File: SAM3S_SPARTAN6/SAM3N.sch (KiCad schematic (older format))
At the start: 28 parts, among them U11 ZLDO1117G33TA, X401 12MHz

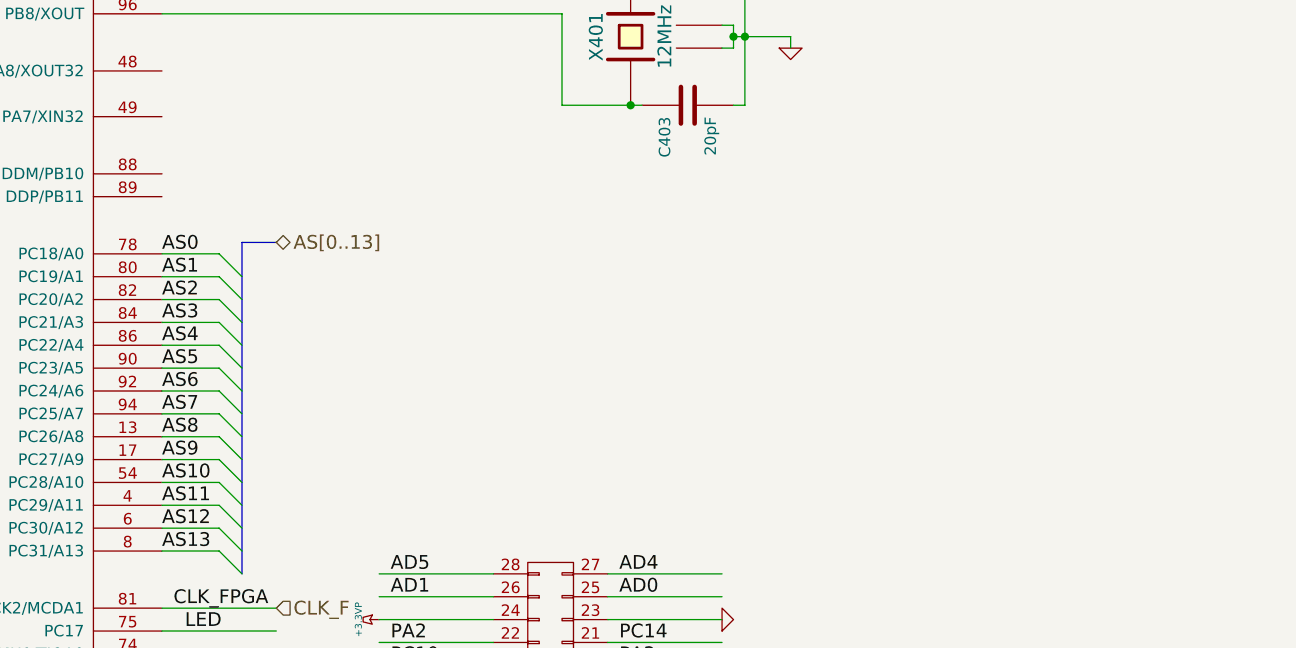
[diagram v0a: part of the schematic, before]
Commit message: Routing
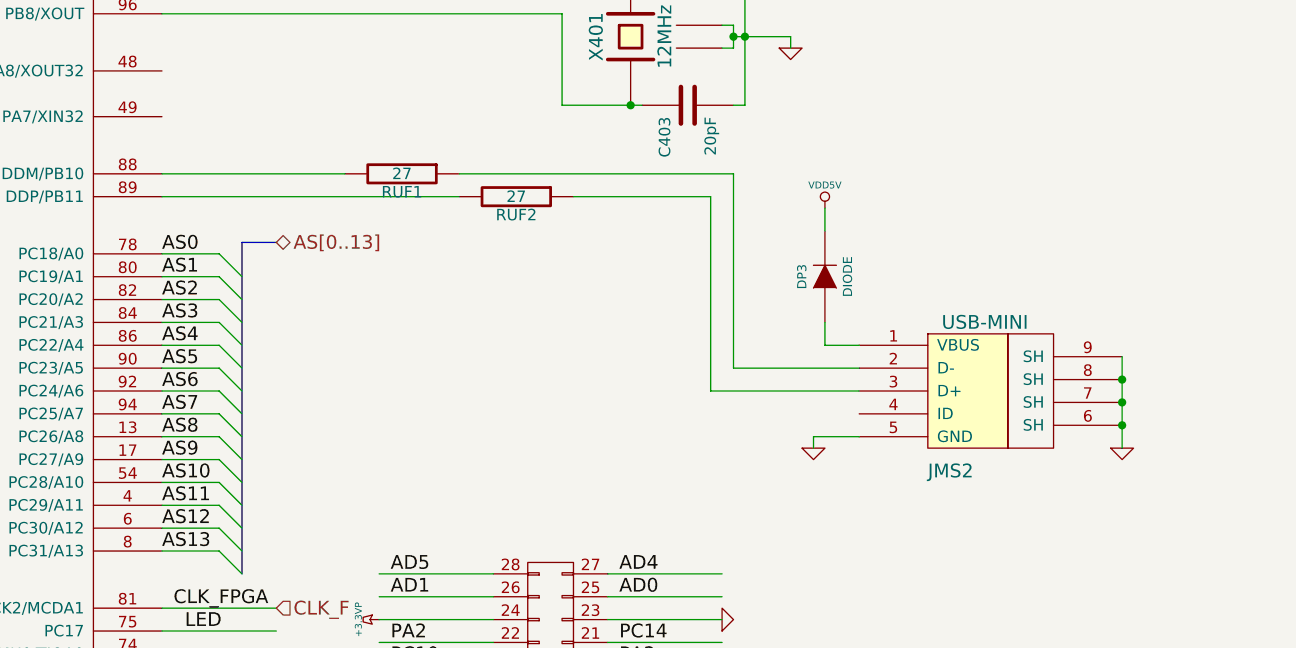
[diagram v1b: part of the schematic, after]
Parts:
- added DP3: DIODE, opendous:SM0603_Opendous, symbol DIODE
- added JMS2: USB-MINI, Connect:USB_Mini-B, symbol USB-MINI
- added RUF1, RUF2: 27, SM0603, symbol R
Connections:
- wire segments 165 -> 180
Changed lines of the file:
@@
 Text HLabel 5400 4600 2    60   Input ~ 0
 CLK_F
+$Comp
+L USB-MINI JMS2
+U 1 1 555B7046
+P 8600 3550
+F 0 "JMS2" H 8350 4000 60  0000 C CNN
+F 1 "USB-MINI" H 8500 3350 60  0000 C CNN
+F 2 "Connect:USB_Mini-B" H 8600 3550 60  0001 C CNN
+F 3 "" H 8600 3550 60  0000 C CNN
+	1    8600 3550
+	1    0    0    1
+$EndComp
+Wire Wire Line
+	7400 3550 7950 3550
+Wire Wire Line
+	7300 3650 7950 3650
+$Comp
+L GND #PWR?
+U 1 1 555B7051
+P 7750 3900
+F 0 "#PWR?" H 7750 3900 30  0001 C CNN
+F 1 "GND" H 7750 3830 30  0001 C CNN
+F 2 "" H 7750 3900 60  0001 C CNN
+F 3 "" H 7750 3900 60  0001 C CNN
+	1    7750 3900
+	1    0    0    -1
+$EndComp
+Wire Wire Line
+	7950 3850 7750 3850
+Wire Wire Line
+	7750 3850 7750 3900
+Wire Wire Line
+	9100 3500 9100 3900
+Connection ~ 9100 3700
+Connection ~ 9100 3600
+$Comp
+L DIODE DP3
+U 1 1 555B705C
+P 7800 3150
+F 0 "DP3" H 7800 3250 40  0000 C CNN
+F 1 "DIODE" H 7800 3050 40  0000 C CNN
+F 2 "opendous:SM0603_Opendous" H 7800 3150 60  0001 C CNN
+F 3 "" H 7800 3150 60  0000 C CNN
+	1    7800 3150
+	0    -1   -1   0
+$EndComp
+$Comp
+L VDD5V #PWR?
+U 1 1 555B7063
+P 7800 2850
+F 0 "#PWR?" H 7800 2950 30  0001 C CNN
+F 1 "VDD5V" H 7800 2950 30  0000 C CNN
+F 2 "" H 7800 2850 60  0001 C CNN
+F 3 "" H 7800 2850 60  0001 C CNN
+	1    7800 2850
+	1    0    0    -1
+$EndComp
+Wire Wire Line
+	7800 2850 7800 2950
+Wire Wire Line
+	7950 3450 7800 3450
+Wire Wire Line
+	7800 3450 7800 3350
+$Comp
+L GND #PWR?
+U 1 1 555B706C
+P 9100 3900
+F 0 "#PWR?" H 9100 3900 30  0001 C CNN
+F 1 "GND" H 9100 3830 30  0001 C CNN
+F 2 "" H 9100 3900 60  0001 C CNN
+F 3 "" H 9100 3900 60  0001 C CNN
+	1    9100 3900
+	1    0    0    -1
+$EndComp
+Connection ~ 9100 3800
+Wire Wire Line
+	7400 2700 7400 3550
+Wire Wire Line
+	7700 3550 7700 3550
+Wire Wire Line
+	7300 3650 7300 2800
+$Comp
+L R RUF1
+U 1 1 555B9831
+P 5950 2700
+F 0 "RUF1" V 6030 2700 50  0000 C CNN
+F 1 "27" V 5950 2700 50  0000 C CNN
+F 2 "SM0603" H 5950 2700 60  0001 C CNN
+F 3 "" H 5950 2700 60  0001 C CNN
+	1    5950 2700
+	0    1    1    0
+$EndComp
+$Comp
+L R RUF2
+U 1 1 555B9AE4
+P 6450 2800
+F 0 "RUF2" V 6530 2800 50  0000 C CNN
+F 1 "27" V 6450 2800 50  0000 C CNN
+F 2 "SM0603" H 6450 2800 60  0001 C CNN
+F 3 "" H 6450 2800 60  0001 C CNN
+	1    6450 2800
+	0    1    1    0
+$EndComp
+Wire Wire Line
+	6200 2700 7400 2700
+Wire Wire Line
+	7300 2800 6700 2800
+Wire Wire Line
+	5700 2700 4900 2700
+Wire Wire Line
+	4900 2800 6200 2800
 $EndSCHEMATC
